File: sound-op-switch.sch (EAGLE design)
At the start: 35 parts, among them IC1 PIC12F1822, IC2 LM358D, T1 MMBTA13

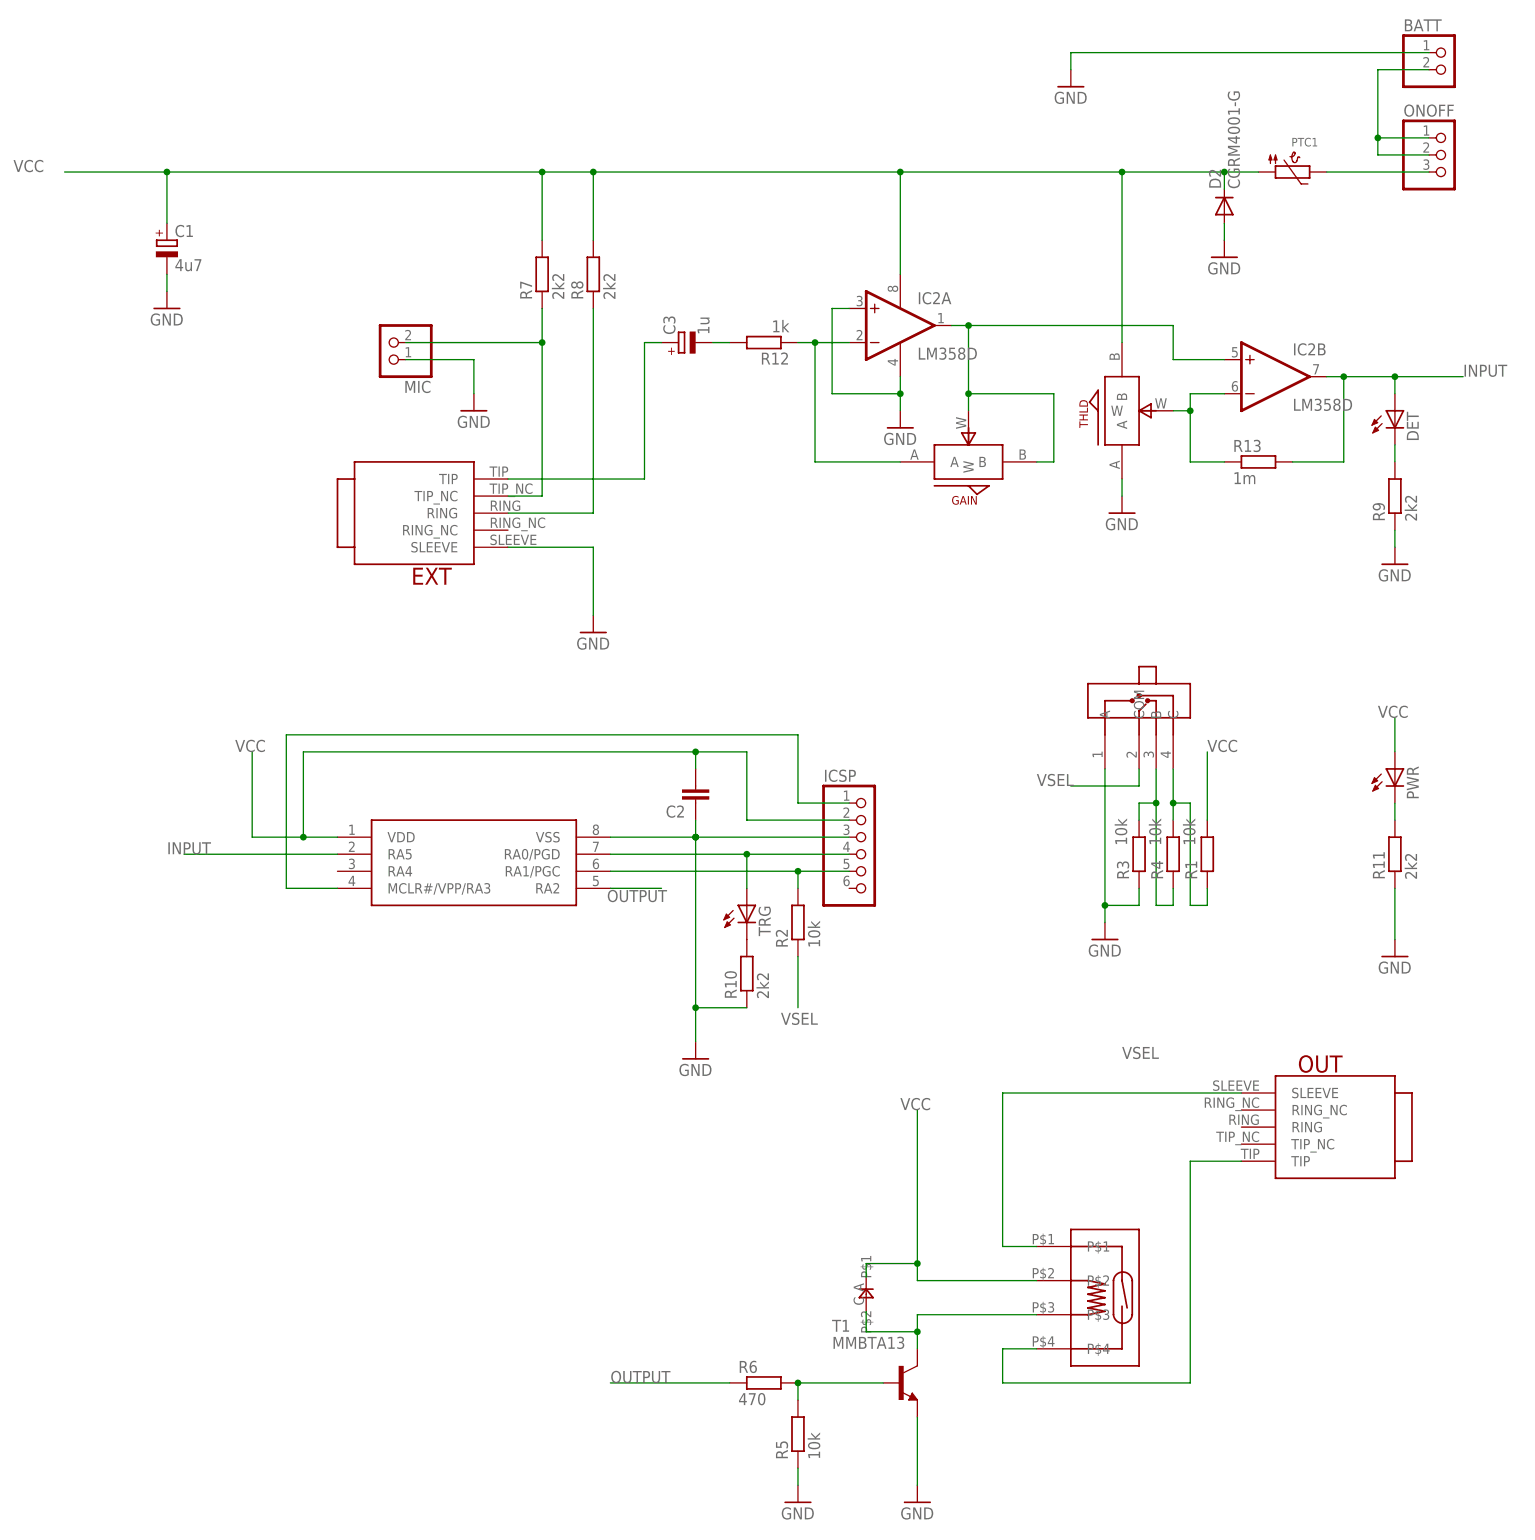
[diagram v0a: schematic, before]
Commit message: pcb rev2
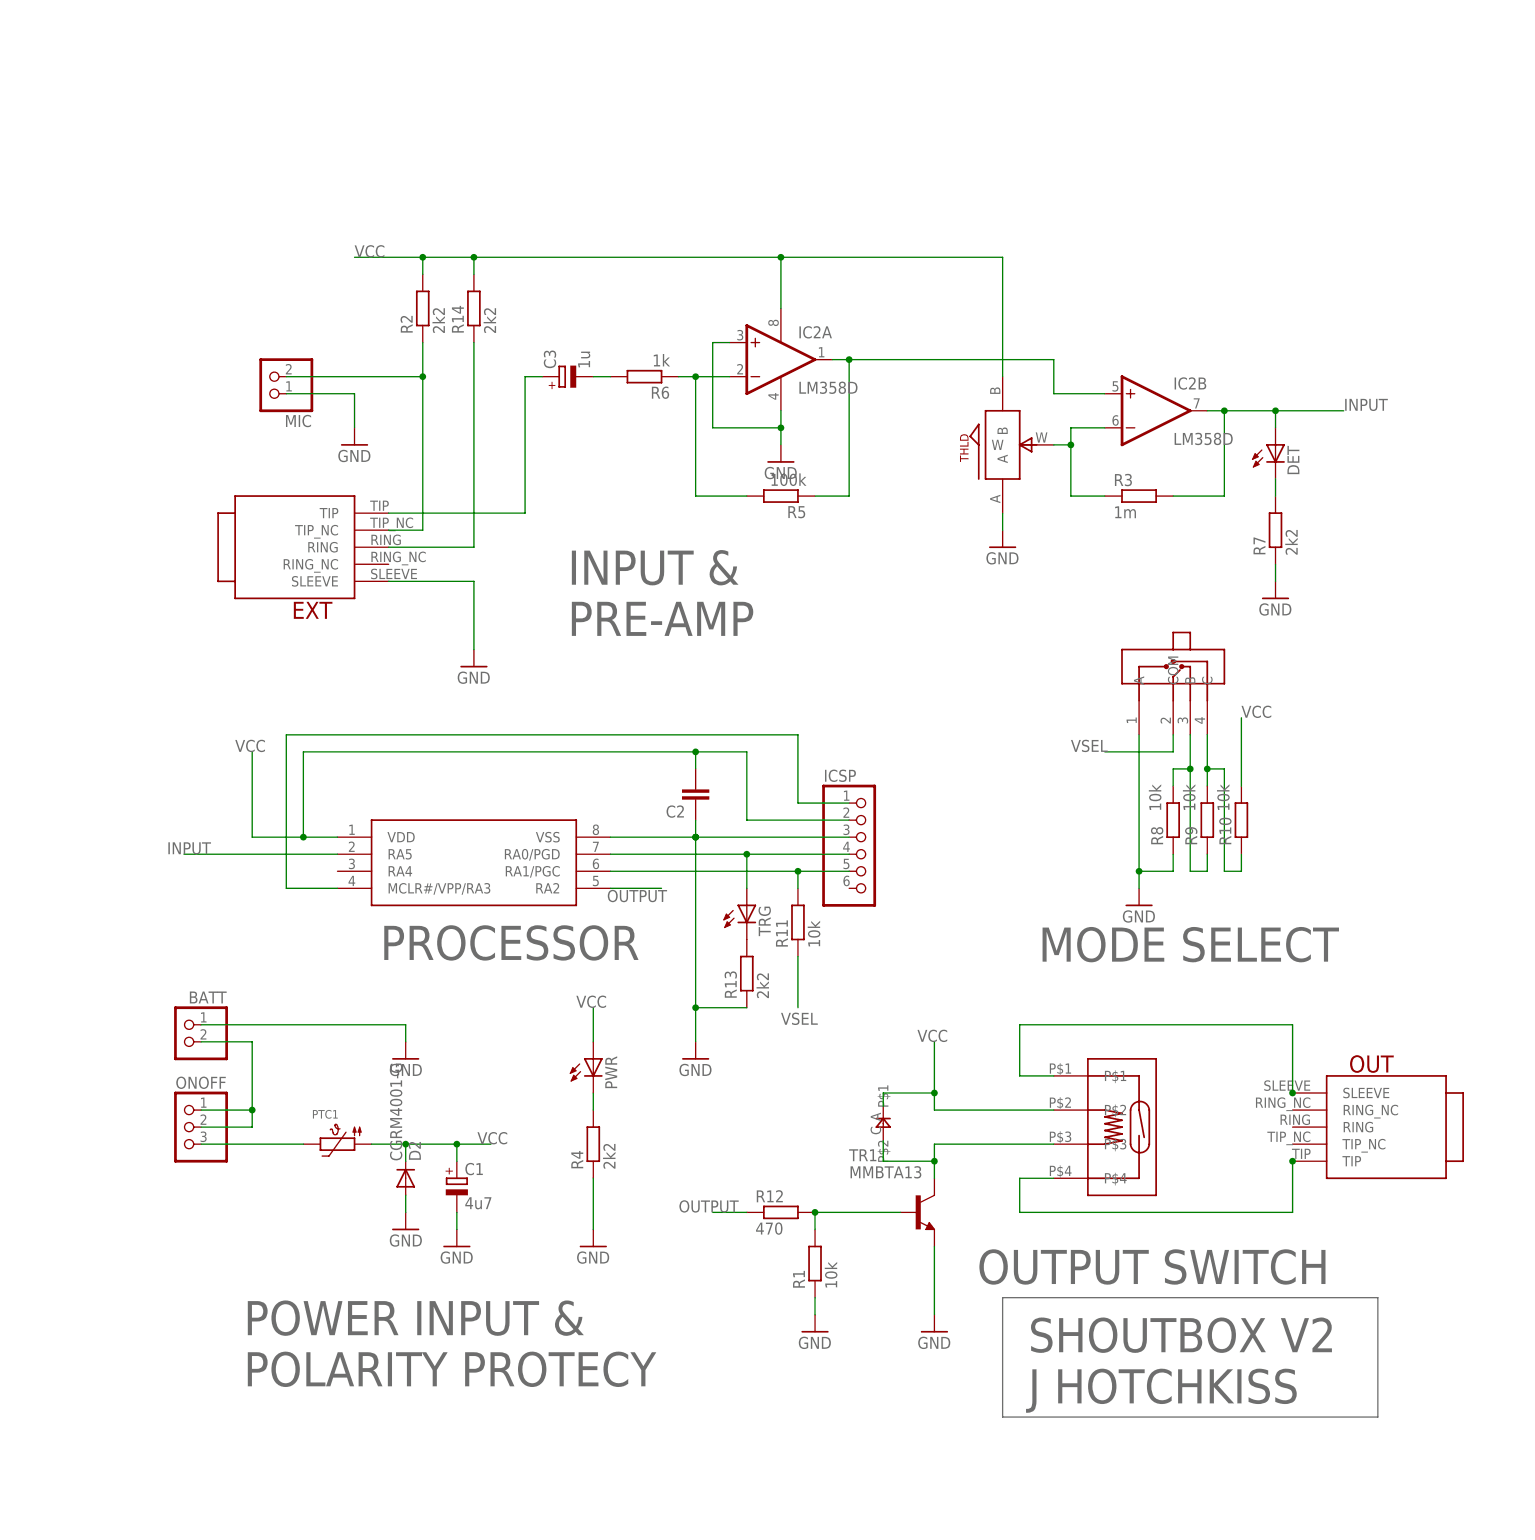
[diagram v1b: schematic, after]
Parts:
- removed GAIN: ALPS_POT_SMALL, jasons_stuff:ALPS_POT_SMALL
- removed MODE: SP4T-SLIDE, jason_eagle6:SP4T-SLIDE
- removed T1: MMBTA13, transistor-neu-to92:MMBT3904LT1-NPN-SOT23-BEC
- added R14: 2k2, resistor:R-EU_R0805
- added SEL: SP4T-SLIDE, jason_eagle6:SP4T-SLIDE
- added TR1: MMBTA13, transistor-neu-to92:MMBT3904LT1-NPN-SOT23-BEC
- R10, R11, R8, R9: value 2k2 -> 10k
- R12: value 1k -> 470; device rcl:R-EU_R0805 -> resistor:R-EU_R0805
- R13: value 1m -> 2k2
- R2, R4: value 10k -> 2k2
- R3: value 10k -> 1m
- R5: value 10k -> 100k; device resistor:R-EU_R0805 -> rcl:R-EU_R0805
- R6: value 470 -> 1k; device resistor:R-EU_R0805 -> rcl:R-EU_R0805
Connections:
- net GND: now also R1.1, R13.1, R4.1, R7.1, R8.1, SEL.A, TR1.E; no longer MODE.A, R10.1, R11.1, R3.1, R5.1, R9.1, T1.E
- net INPUT: now also R3.2; no longer R13.2
- net N$1: now also R2.1; no longer R7.1
- net N$10: now also R1.2, R12.2, TR1.B; no longer R5.2, R6.2, T1.B
- net N$13: now also R3.1; no longer R13.1
- net N$14: now also R8.2, R9.1, SEL.B; no longer MODE.B, R3.2, R4.1
- net N$15: now also TR1.C; no longer T1.C
- net N$16: now also R4.2; no longer R11.2
- net N$17: now also R13.2; no longer R10.2
- net N$2: now also R6.2; no longer R12.2
- net N$3: now also R5.2, R6.1; no longer GAIN.A, R12.1
- net N$4: now also R7.2; no longer R9.2
- net N$5: now also R14.1; no longer R8.1
- net N$7: now also R5.1; no longer GAIN.B, GAIN.W
- net N$8: now also R10.1, R9.2, SEL.C; no longer MODE.C, R1.1, R4.2
- net N$9: now also R11.2; no longer R2.2
- net OUTPUT: now also R12.1; no longer R6.1
- net VCC: now also R10.2, R14.2, R2.2; no longer R1.2, R7.2, R8.2
- net VSEL: now also R11.1, SEL.COM; no longer MODE.COM, R2.1
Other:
- note added: "INPUT & PRE-AMP"
- note added: "J HOTCHKISS"
- note added: "MODE SELECT"
- note added: "OUTPUT SWITCH"
- note added: "POWER INPUT & POLARITY PROTECY"
- note added: "PROCESSOR"
- note added: "SHOUTBOX V2"
- moved on the sheet: BATT, C1, C3, D2, DET, EXT, IC2A, IC2B, MIC, ONOFF, OUT, PTC1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
